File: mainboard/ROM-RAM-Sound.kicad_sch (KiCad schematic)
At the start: 13 parts, among them J5 ROM Select, J6 ROM Select, J7 Sound Clock Select, J8 AUDIO OUT, U29 HM62256BLP, U30 HM62256BLP, U31 27C64, U32 27C64, U33 SN76489

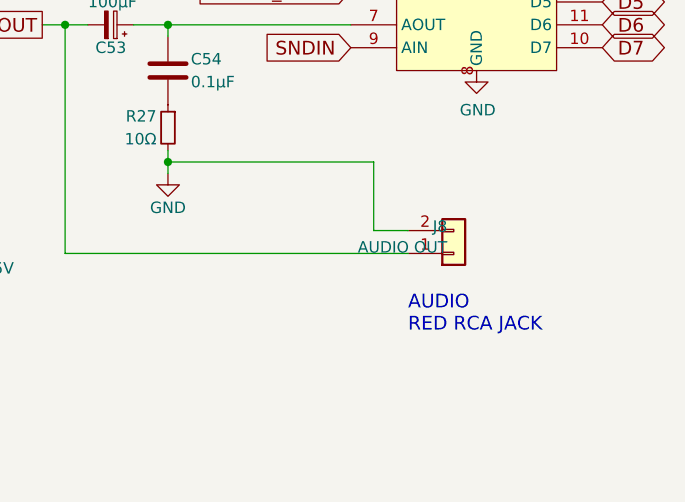
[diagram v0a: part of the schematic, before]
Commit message: layout work
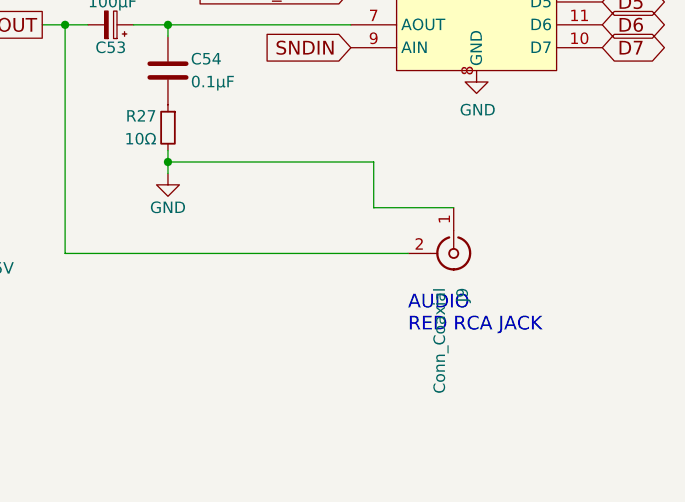
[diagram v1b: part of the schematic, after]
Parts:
- removed J8: AUDIO OUT, Custom:STD_DDW_PINHEAD_V_1x02, symbol Connector_Generic:Conn_01x02
- added J9: Conn_Coaxial, Custom:CUI_RCJ-047, symbol Connector:Conn_Coaxial
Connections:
- net GND: now also J9.1 (In)
- net SNDOUT: now also J9.2 (Ext)
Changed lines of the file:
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@@
 	(wire
 		(pts
-			(xy 224.79 125.73) (xy 224.79 118.11)
-		)
-		(stroke
-			(width 0)
-			(type default)
-		)
-	)
-	(wire
-		(pts
 			(xy 201.93 116.84) (xy 201.93 118.11)
 		)
@@
 	(wire
 		(pts
+			(xy 224.79 123.19) (xy 233.68 123.19)
+		)
+		(stroke
+			(width 0)
+			(type default)
+		)
+	)
+	(wire
+		(pts
 			(xy 52.07 132.08) (xy 52.07 135.89)
 		)
@@
 	(wire
 		(pts
-			(xy 228.6 125.73) (xy 224.79 125.73)
-		)
-		(stroke
-			(width 0)
-			(type default)
-		)
-	)
-	(wire
-		(pts
 			(xy 124.46 106.68) (xy 127 106.68)
 		)
@@
 	(wire
 		(pts
+			(xy 224.79 123.19) (xy 224.79 118.11)
+		)
+		(stroke
+			(width 0)
+			(type default)
+		)
+	)
+	(wire
+		(pts
 			(xy 81.28 53.34) (xy 81.28 57.15)
 		)
@@
 	)
 	(symbol
+		(lib_id "Connector:Conn_Coaxial")
+		(at 233.68 128.27 270)
+		(unit 1)
+		(exclude_from_sim no)
+		(in_bom yes)
+		(on_board yes)
+		(dnp no)
+		(property "Reference" "J9"
+			(at 234.6569 132.08 0)
+			(effects
+				(font
+					(size 1.27 1.27)
+				)
+				(justify left)
+			)
+		)
+		(property "Value" "Conn_Coaxial"
+			(at 232.1169 132.08 0)
+			(effects
+				(font
+					(size 1.27 1.27)
+				)
+				(justify left)
+			)
+		)
+		(property "Footprint" "Custom:CUI_RCJ-047"
+			(at 233.68 128.27 0)
+			(effects
+				(font
+					(size 1.27 1.27)
+				)
+				(hide yes)
+			)
+		)
+		(property "Datasheet" "~"
+			(at 233.68 128.27 0)
+			(effects
+				(font
+					(size 1.27 1.27)
+				)
+				(hide yes)
+			)
+		)
+		(property "Description" "coaxial connector (BNC, SMA, SMB, SMC, Cinch/RCA, LEMO, ...)"
+			(at 233.68 128.27 0)
+			(effects
+				(font
+					(size 1.27 1.27)
+				)
+				(hide yes)
+			)
+		)
+		(pin "1"
+		)
+		(pin "2"
+		)
+		(instances
+			(project "Console"
+				(path "/10b20c6b-8045-46d1-a965-0d7dd9a1b5fa/00000000-0000-0000-0000-0000561cdf3b"
+					(reference "J9")
+					(unit 1)
+				)
+			)
+		)
+	)
+	(symbol
 		(lib_id "power:+5V")
 		(at 127 83.82 270)
@@
 					(unit 1)
 				)
-			)
-		)
-	)
-	(symbol
-		(lib_id "Connector_Generic:Conn_01x02")
-		(at 233.68 128.27 0)
-		(mirror x)
-		(unit 1)
-		(exclude_from_sim no)
-		(in_bom yes)
-		(on_board yes)
-		(dnp no)
-		(property "Reference" "J8"
-			(at 232.9688 125.2728 0)
-			(effects
-				(font
-					(size 1.27 1.27)
-				)
-				(justify right)
-			)
-		)
-		(property "Value" "AUDIO OUT"
-			(at 232.9688 127.5842 0)
-			(effects
-				(font
-					(size 1.27 1.27)
-				)
-				(justify right)
-			)
-		)
-		(property "Footprint" "Custom:STD_DDW_PINHEAD_V_1x02"
-			(at 233.68 128.27 0)
-			(effects
-				(font
-					(size 1.27 1.27)
-				)
-				(hide yes)
-			)
-		)
-		(property "Datasheet" "~"
-			(at 233.68 128.27 0)
-			(effects
-				(font
-					(size 1.27 1.27)
-				)
-				(hide yes)
-			)
-		)
-		(property "Description" "Generic connector, single row, 01x02, script generated (kicad-library-utils/schlib/autogen/connector/)"
-			(at 233.68 128.27 0)
-			(effects
-				(font
-					(size 1.27 1.27)
-				)
-				(hide yes)
-			)
-		)
-		(pin "1"
-		)
-		(pin "2"
-		)
-		(instances
-			(project ""
-				(path "/10b20c6b-8045-46d1-a965-0d7dd9a1b5fa/00000000-0000-0000-0000-0000561cdf3b"
-					(reference "J8")
-					(unit 1)
-				)
